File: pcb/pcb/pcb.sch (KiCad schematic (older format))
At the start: 40 parts, among them J102 Barrel_Jack, J103 Conn_01x07, J105 Conn_01x07, J106 Conn_01x07, J107 Conn_01x07, J108 Conn_01x07, J109 Conn_01x07, J11 Conn_01x34, J111 Conn_01x07, J112 Conn_01x07, J113 Conn_01x07, J12 Conn_01x12, J13 Conn_01x03, J14 DIN-5_180degree, J15 DIN-5_180degree, SW1 SW_Push, U1 74HC595, U2 6N137, U3 MCP4811, U4 LM324

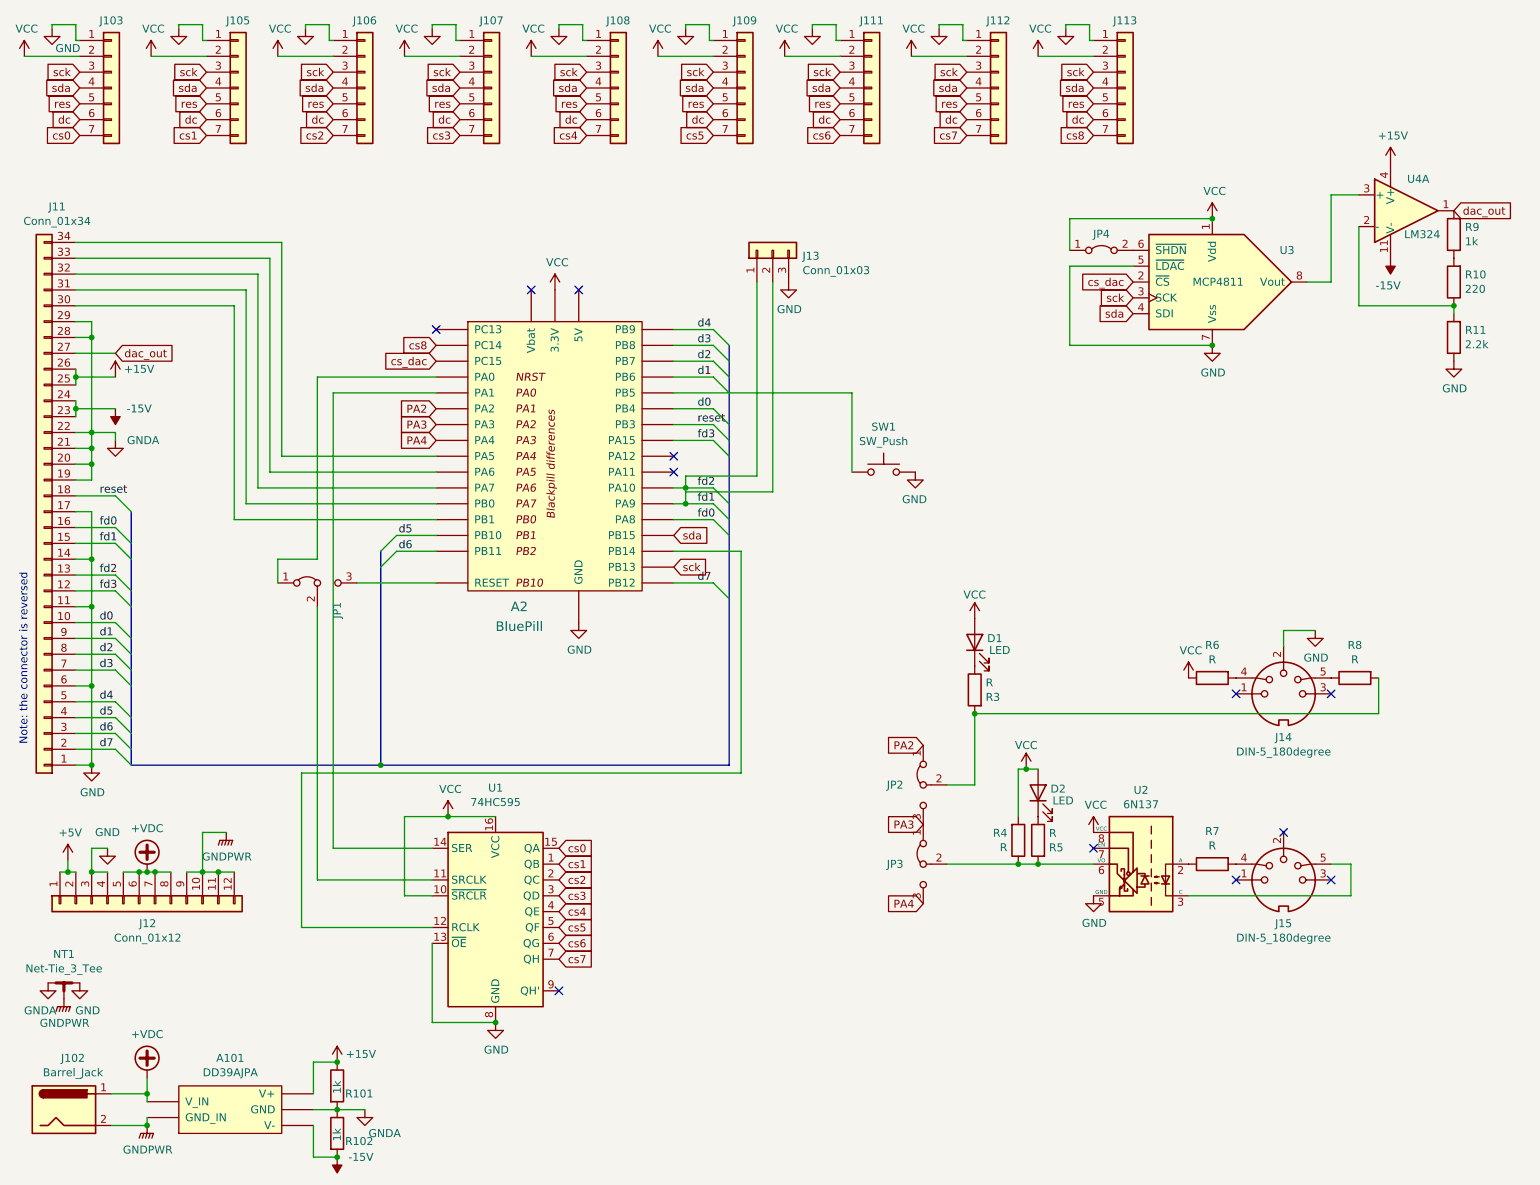
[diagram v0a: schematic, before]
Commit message: pcb++
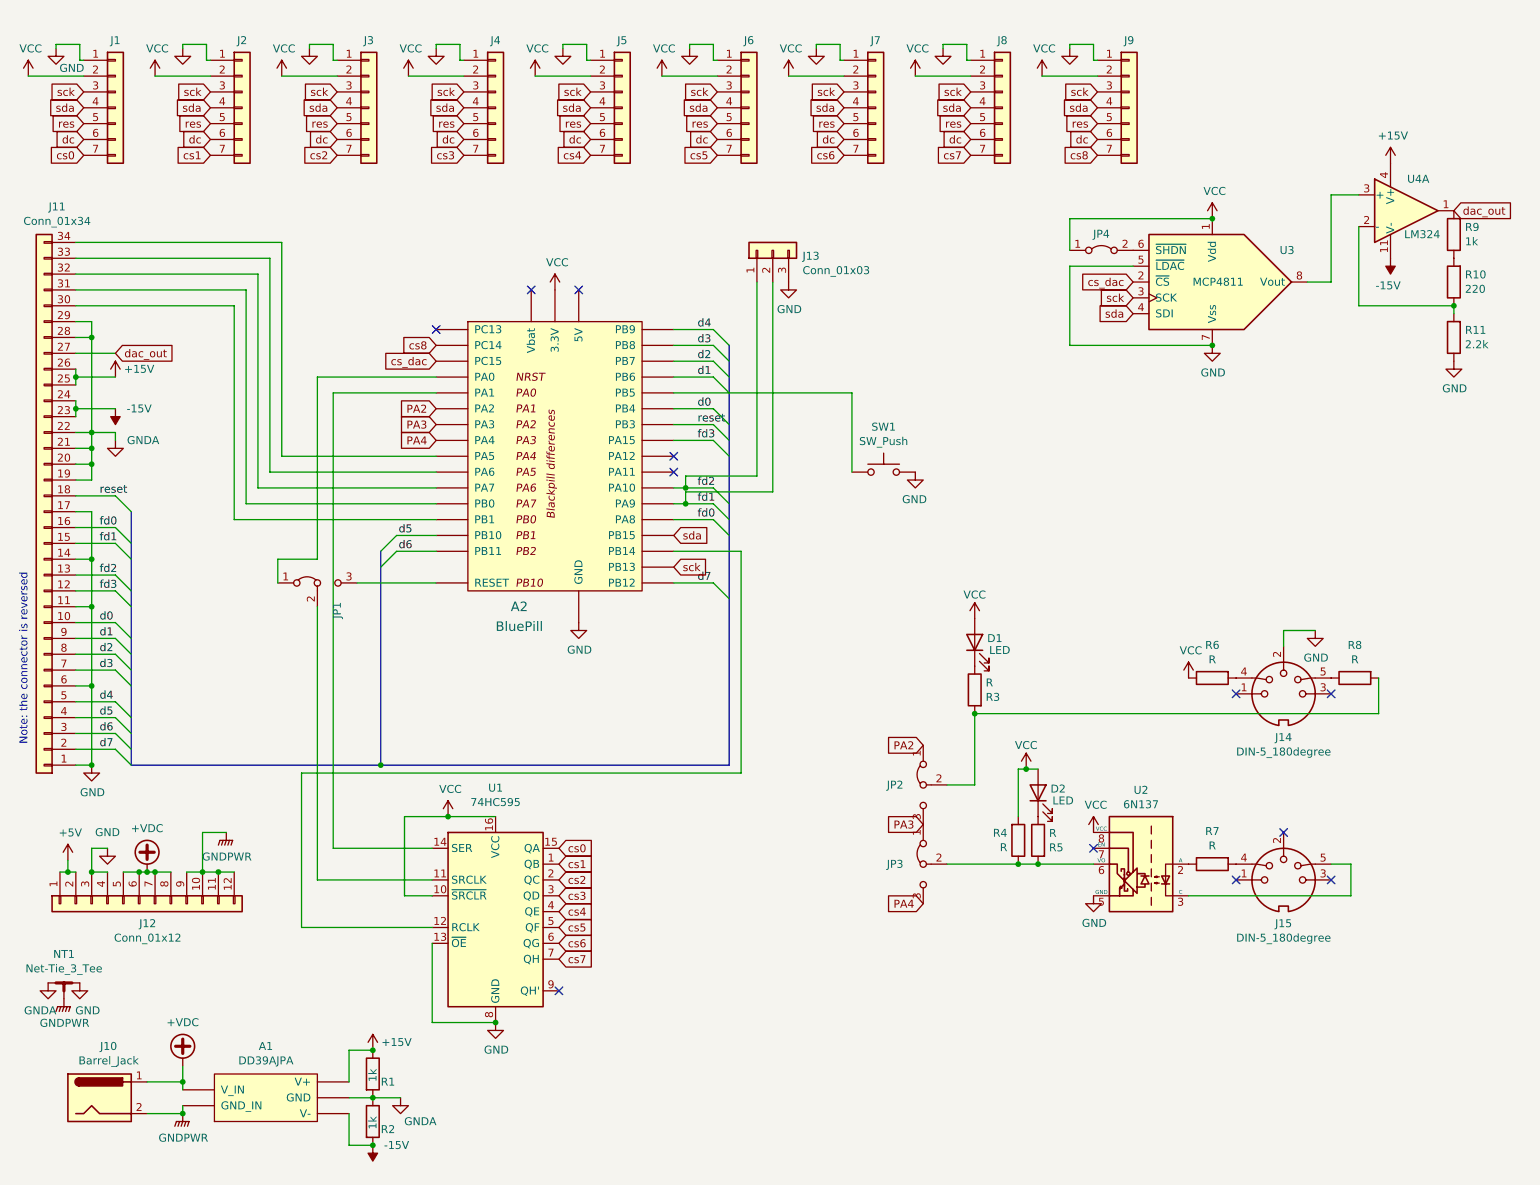
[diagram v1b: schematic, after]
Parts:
- J13: footprint Connector_JST:JST_XH_B7B-XH-A_1x07_P2.50mm_Vertical -> Connector_PinHeader_2.54mm:PinHeader_1x03_P2.54mm_Horizontal
- renumbered A101 to A1, J103 to J1, J102 to J10, J105 to J2, J106 to J3, J107 to J4, J108 to J5, J109 to J6, J111 to J7, J112 to J8, J113 to J9, R101 to R1, R102 to R2
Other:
- moved on the sheet: A1, J1, J10, J2, J3, J4, J5, J6, J7, J8, J9, R1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
